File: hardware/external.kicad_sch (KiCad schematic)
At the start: 5 parts, among them J1 BASYS3, U1 MCP4728

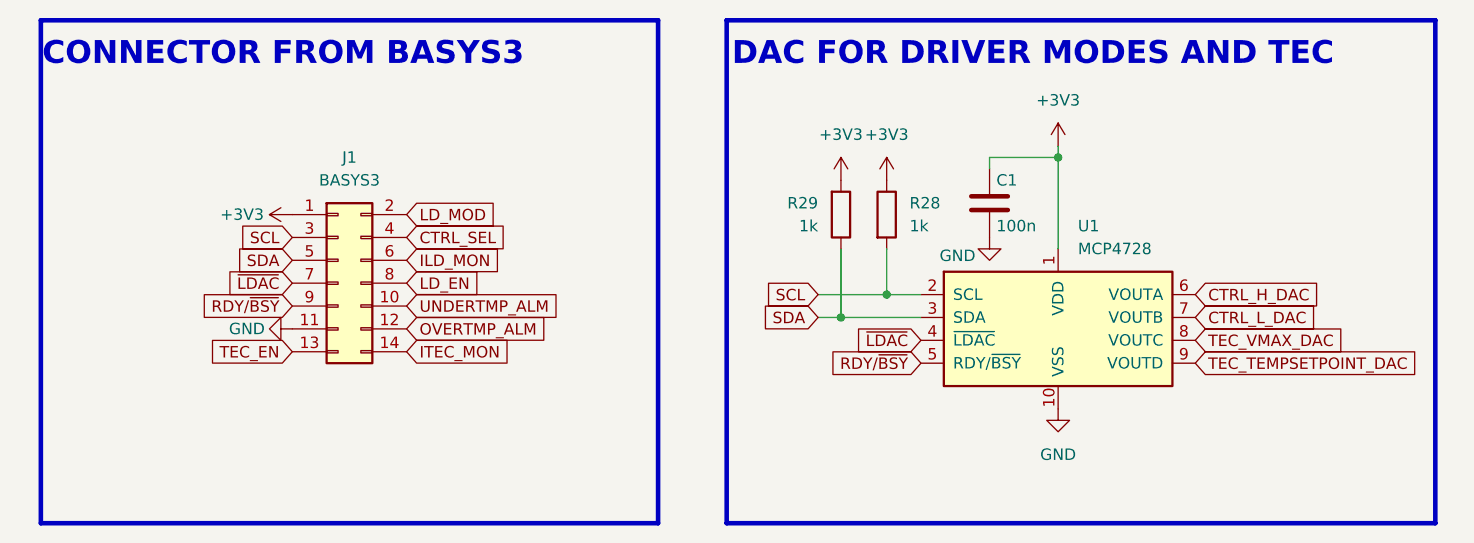
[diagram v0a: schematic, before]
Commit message: feat: decent readme as user manual
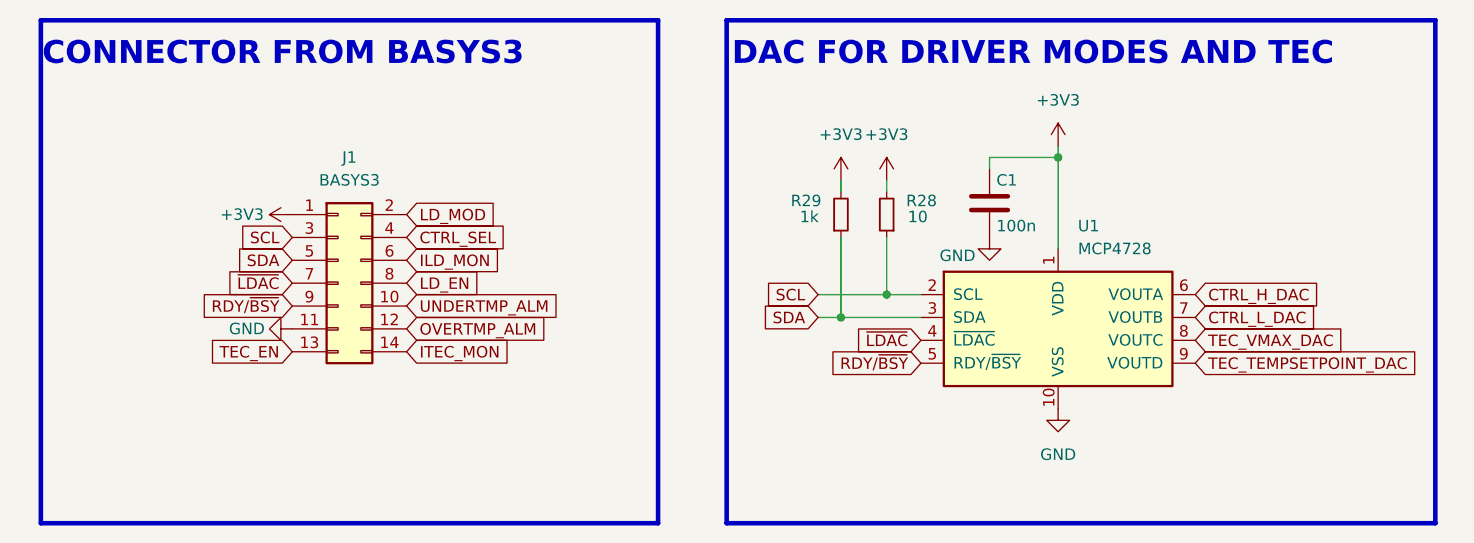
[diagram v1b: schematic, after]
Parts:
- removed R28, R29: 1k, symbol Device:R
- added R28: 10, Resistor_SMD:R_0603_1608Metric, symbol Device:R_Small
- added R29: 1k, Resistor_SMD:R_0603_1608Metric, symbol Device:R_Small
- J1: footprint Connector_PinHeader_2.54mm:PinHeader_2x07_P2.54mm_Horizontal -> Connector_PinHeader_2.54mm:PinHeader_2x07_P2.54mm_Vertical
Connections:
- net +3V3: now also R28.2, R29.2
- net SCL: now also R28.1
- net SDA: now also R29.1
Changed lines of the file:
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@@
 	(wire
 		(pts
-			(xy 160.02 93.98) (xy 160.02 101.6)
+			(xy 176.53 83.82) (xy 176.53 85.09)
 		)
 		(stroke
@@
 	(wire
 		(pts
-			(xy 176.53 83.82) (xy 176.53 85.09)
+			(xy 160.02 86.36) (xy 160.02 87.63)
 		)
 		(stroke
@@
 	(wire
 		(pts
-			(xy 165.1 93.98) (xy 165.1 99.06)
+			(xy 165.1 86.36) (xy 165.1 87.63)
 		)
 		(stroke
@@
 		)
 	)
+	(wire
+		(pts
+			(xy 165.1 92.71) (xy 165.1 99.06)
+		)
+		(stroke
+			(width 0)
+			(type default)
+		)
+	)
 	(polyline
 		(pts
@@
 		(pts
 			(xy 184.15 83.82) (xy 184.15 93.98)
+		)
+		(stroke
+			(width 0)
+			(type default)
+		)
+	)
+	(wire
+		(pts
+			(xy 160.02 92.71) (xy 160.02 101.6)
 		)
 		(stroke
@@
 	)
 	(symbol
-		(lib_id "Device:R")
-		(at 165.1 90.17 0)
+		(lib_id "Device:R_Small")
+		(at 165.1 90.17 180)
 		(unit 1)
 		(exclude_from_sim no)
@@
 		(on_board yes)
 		(dnp no)
-		(fields_autoplaced yes)
 		(property "Reference" "R28"
-			(at 167.64 88.8999 0)
-			(effects
-				(font
-					(size 1.27 1.27)
-				)
-				(justify left)
-			)
-		)
-		(property "Value" "1k"
-			(at 167.64 91.4399 0)
-			(effects
-				(font
-					(size 1.27 1.27)
-				)
-				(justify left)
-			)
-		)
-		(property "Footprint" ""
-			(at 163.322 90.17 90)
+			(at 170.688 88.646 0)
+			(effects
+				(font
+					(size 1.27 1.27)
+				)
+				(justify left)
+			)
+		)
+		(property "Value" "10"
+			(at 169.672 90.424 0)
+			(effects
+				(font
+					(size 1.27 1.27)
+				)
+				(justify left)
+			)
+		)
+		(property "Footprint" "Resistor_SMD:R_0603_1608Metric"
+			(at 165.1 90.17 0)
 			(effects
 				(font
@@
 			)
 		)
-		(property "Description" "Resistor"
+		(property "Description" "Resistor, small symbol"
 			(at 165.1 90.17 0)
 			(effects
@@
 			)
 		)
+		(property "Sim.Device" ""
+			(at 165.1 90.17 0)
+			(effects
+				(font
+					(size 1.27 1.27)
+				)
+				(hide yes)
+			)
+		)
+		(property "Sim.Pins" ""
+			(at 165.1 90.17 0)
+			(effects
+				(font
+					(size 1.27 1.27)
+				)
+				(hide yes)
+			)
+		)
+		(property "Sim.Type" ""
+			(at 165.1 90.17 0)
+			(effects
+				(font
+					(size 1.27 1.27)
+				)
+				(hide yes)
+			)
+		)
+		(property "PN" "CRCW060310R0FKEAC "
+			(at 165.1 90.17 0)
+			(effects
+				(font
+					(size 1.27 1.27)
+				)
+				(hide yes)
+			)
+		)
+		(property "Store Link" "https://www.mouser.it/ProductDetail/Vishay-Dale/CRCW060310R0FKEAC?qs=E3Y5ESvWgWP5XvJ40P8QAg%3D%3D"
+			(at 165.1 90.17 0)
+			(effects
+				(font
+					(size 1.27 1.27)
+				)
+				(hide yes)
+			)
+		)
 		(pin "2"
 		)
@@
 		)
 		(instances
-			(project ""
+			(project "SOA-driver"
 				(path "/aef12ca3-3d60-44eb-99b6-8bdd18a4b35c/b8096563-2aa1-42a7-b303-2d7d794c80ce"
 					(reference "R28")
@@
 	)
 	(symbol
-		(lib_id "Device:R")
+		(lib_id "Device:R_Small")
 		(at 160.02 90.17 0)
 		(mirror x)
@@
 		(on_board yes)
 		(dnp no)
-		(fields_autoplaced yes)
 		(property "Reference" "R29"
-			(at 157.48 88.8999 0)
-			(effects
-				(font
-					(size 1.27 1.27)
-				)
-				(justify right)
+			(at 154.432 88.646 0)
+			(effects
+				(font
+					(size 1.27 1.27)
+				)
+				(justify left)
 			)
 		)
 		(property "Value" "1k"
-			(at 157.48 91.4399 0)
-			(effects
-				(font
-					(size 1.27 1.27)
-				)
-				(justify right)
-			)
-		)
-		(property "Footprint" ""
-			(at 158.242 90.17 90)
+			(at 155.448 90.424 0)
+			(effects
+				(font
+					(size 1.27 1.27)
+				)
+				(justify left)
+			)
+		)
+		(property "Footprint" "Resistor_SMD:R_0603_1608Metric"
+			(at 160.02 90.17 0)
 			(effects
 				(font
@@
 			)
 		)
-		(property "Description" "Resistor"
+		(property "Description" "Resistor, small symbol"
 			(at 160.02 90.17 0)
 			(effects
@@
 			)
 		)
+		(property "Sim.Device" ""
+			(at 160.02 90.17 0)
+			(effects
+				(font
+					(size 1.27 1.27)
+				)
+				(hide yes)
+			)
+		)
+		(property "Sim.Pins" ""
+			(at 160.02 90.17 0)
+			(effects
+				(font
+					(size 1.27 1.27)
+				)
+				(hide yes)
+			)
+		)
+		(property "Sim.Type" ""
+			(at 160.02 90.17 0)
+			(effects
+				(font
+					(size 1.27 1.27)
+				)
+				(hide yes)
+			)
+		)
+		(property "PN" "CRCW060310R0FKEAC "
+			(at 160.02 90.17 0)
+			(effects
+				(font
+					(size 1.27 1.27)
+				)
+				(hide yes)
+			)
+		)
+		(property "Store Link" "https://www.mouser.it/ProductDetail/Vishay-Dale/CRCW060310R0FKEAC?qs=E3Y5ESvWgWP5XvJ40P8QAg%3D%3D"
+			(at 160.02 90.17 0)
+			(effects
+				(font
+					(size 1.27 1.27)
+				)
+				(hide yes)
+			)
+		)
 		(pin "2"
 		)
@@
 		)
 		(instances
-			(project ""
+			(project "SOA-driver"
 				(path "/aef12ca3-3d60-44eb-99b6-8bdd18a4b35c/b8096563-2aa1-42a7-b303-2d7d794c80ce"
 					(reference "R29")
@@
 			)
 		)
-		(property "Footprint" "Connector_PinHeader_2.54mm:PinHeader_2x07_P2.54mm_Horizontal"
+		(property "Footprint" "Connector_PinHeader_2.54mm:PinHeader_2x07_P2.54mm_Vertical"
 			(at 104.14 97.79 0)
 			(effects
